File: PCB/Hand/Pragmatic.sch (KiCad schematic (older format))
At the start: 76 parts, among them J1 Conn_02x08_Odd_Even, J2 Conn_01x04, SW1 SW_Push, SW10 SW_Push, SW11 SW_Push, SW12 SW_Push, SW13 SW_Push, SW14 SW_Push, SW15 SW_Push, SW16 SW_Push, SW17 SW_Push, SW18 SW_Push, SW19 SW_Push, SW2 SW_Push, SW20 SW_Push, SW21 SW_Push, SW22 SW_Push, SW23 SW_Push, SW24 SW_Push, SW25 SW_Push, SW26 SW_Push, SW27 SW_Push, SW28 SW_Push, SW29 SW_Push, SW3 SW_Push, SW30 SW_Push, SW31 SW_Push, SW32 SW_Push, SW33 SW_Push, SW34 SW_Push, SW35 SW_Push, SW36 SW_Push, SW4 SW_Push, SW5 SW_Push, SW6 SW_Push, SW7 SW_Push, SW8 SW_Push, SW9 SW_Push

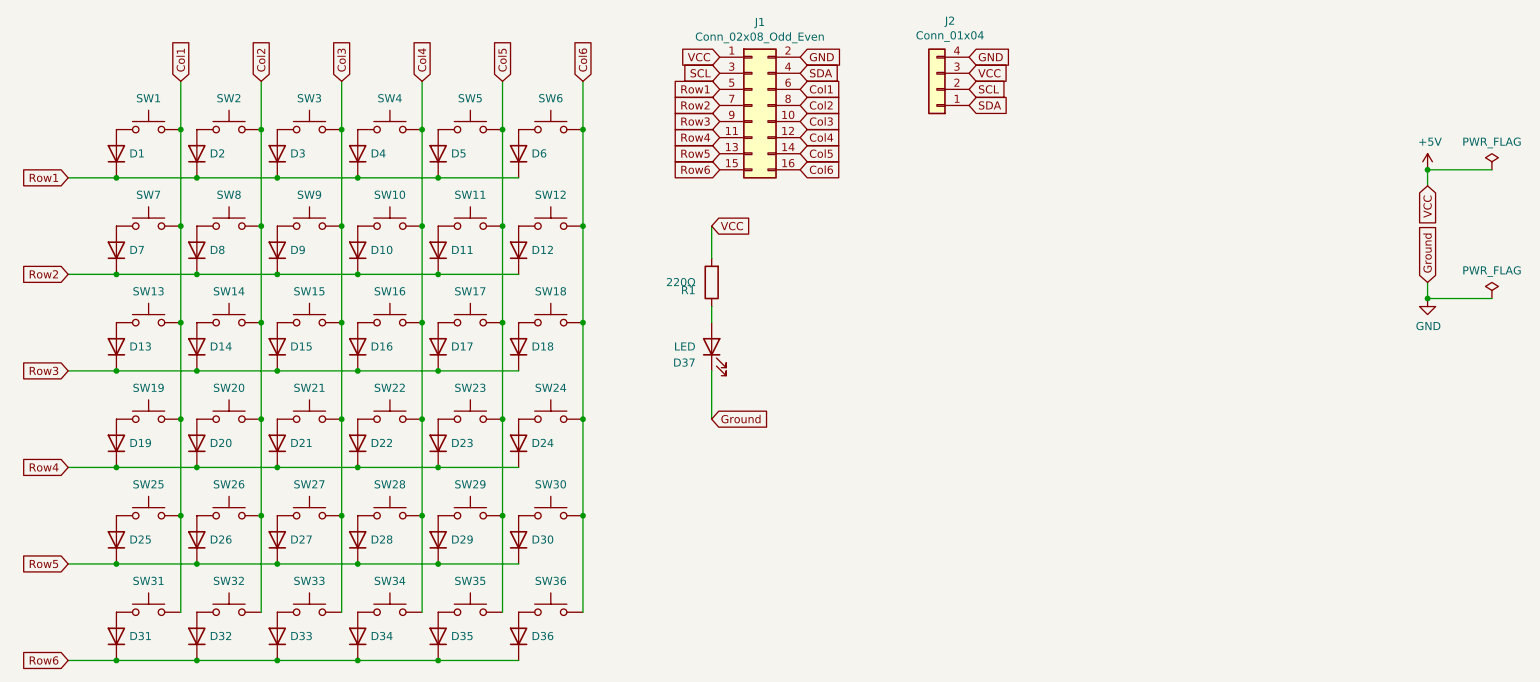
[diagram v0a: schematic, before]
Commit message: double side design
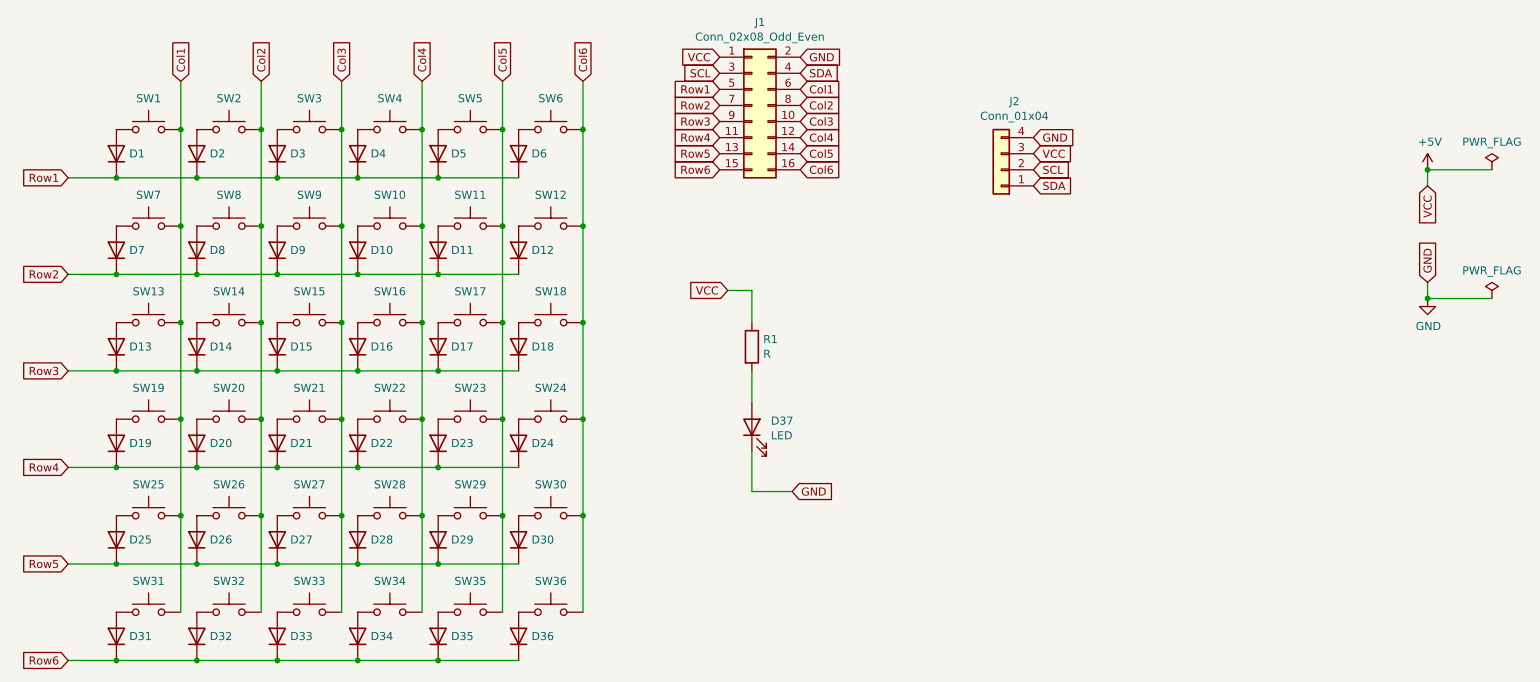
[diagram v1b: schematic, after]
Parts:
- D1, D10, D11, D12, D13, D14, D15, D16, D17, D18, D19, D2, D20, D21, D22, D23, D24, D25, D26, D27, D28, D29, D3, D30, D31, D32, D33, D34, D35, D36, D4, D5, D6, D7, D8, D9: footprint Pragmatic:D_SMD -> Pragmatic:D_SMD_With_Shadow; LCSC (none) -> C81598
- D37: footprint LED_SMD:LED_0805_2012Metric_Pad1.15x1.40mm_HandSolder -> Pragmatic:LED_0805_With_Shadow; LCSC (none) -> C2297
- J1: LCSC (none) -> C3406
- R1: value 220Ω -> R; footprint Resistor_SMD:R_0805_2012Metric_Pad1.20x1.40mm_HandSolder -> Pragmatic:R_0805_With_Shadow; LCSC (none) -> C17408
- SW1, SW10, SW11, SW12, SW13, SW14, SW15, SW16, SW17, SW18, SW19, SW2, SW20, SW21, SW22, SW23, SW24, SW25, SW26, SW27, SW28, SW29, SW3, SW30, SW31, SW32, SW33, SW34, SW35, SW36, SW4, SW5, SW6, SW7, SW8, SW9: footprint Pragmatic:CherryMX_ChocV2_1u -> Pragmatic:Switch_1u_Mirrored
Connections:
- net +5V: now also R1.1; no longer R1.2
- net at D37.2 (A): now also R1.2; no longer R1.1
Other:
- moved on the sheet: J2

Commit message: left hand done.
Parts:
- J2: footprint kbd:OLED -> Connector_PinHeader_2.54mm:PinHeader_1x04_P2.54mm_Vertical
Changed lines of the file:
@@
 F 0 "J2" H 7418 2825 50  0000 C CNN
 F 1 "Conn_01x04" H 7418 2916 50  0000 C CNN
-F 2 "kbd:OLED" H 7500 3250 50  0001 C CNN
+F 2 "Connector_PinHeader_2.54mm:PinHeader_1x04_P2.54mm_Vertical" H 7500 3250 50  0001 C CNN
 F 3 "~" H 7500 3250 50  0001 C CNN
 	1    7500 3250
